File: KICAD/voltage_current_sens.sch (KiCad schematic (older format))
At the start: 22 parts

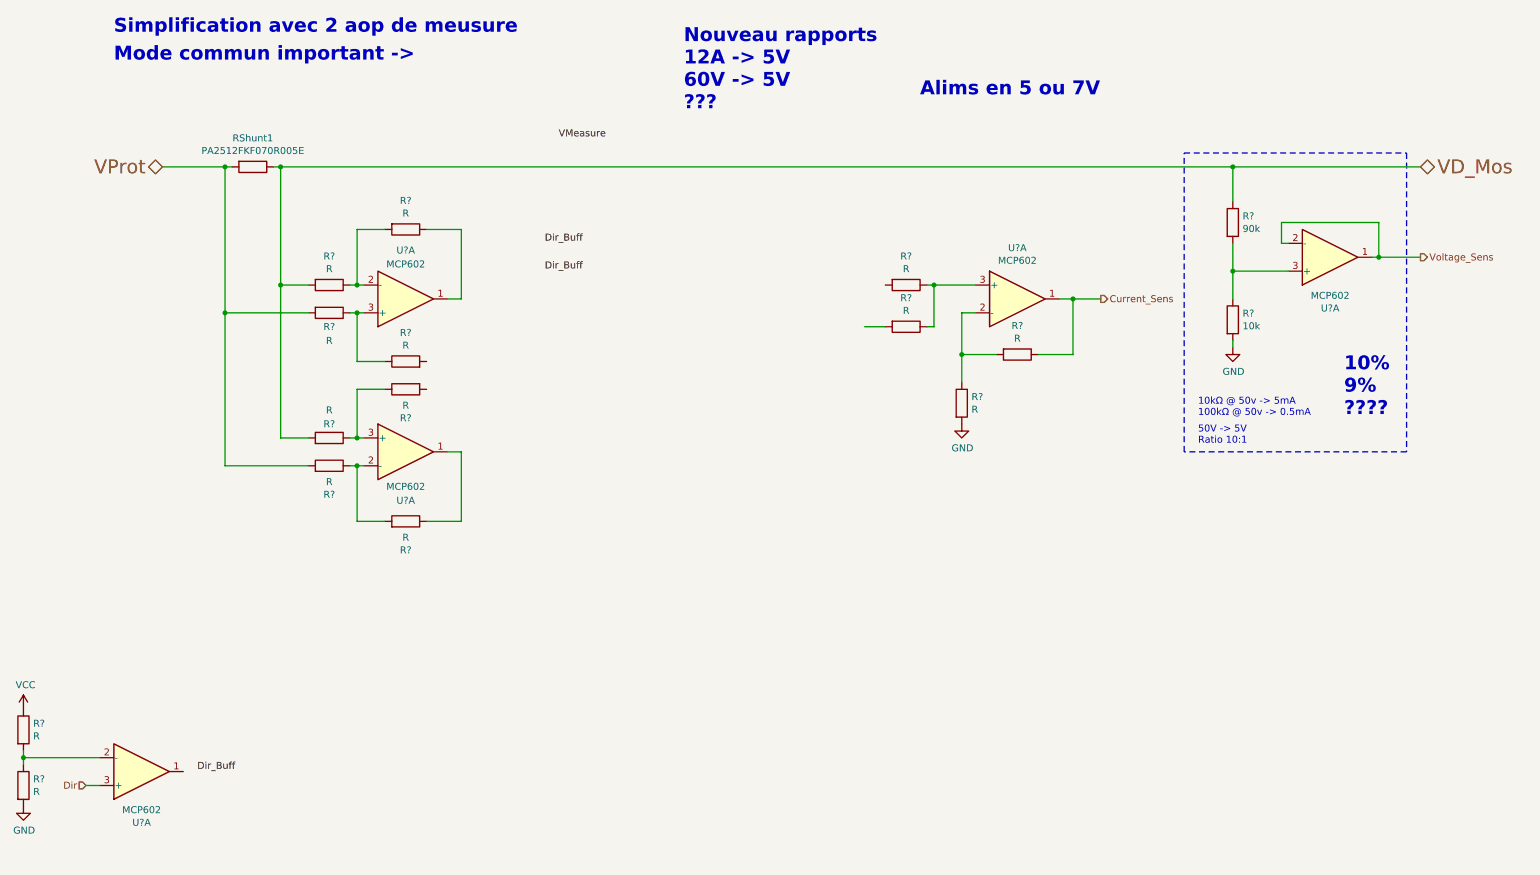
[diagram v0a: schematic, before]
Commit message: worked on power supply + connectors
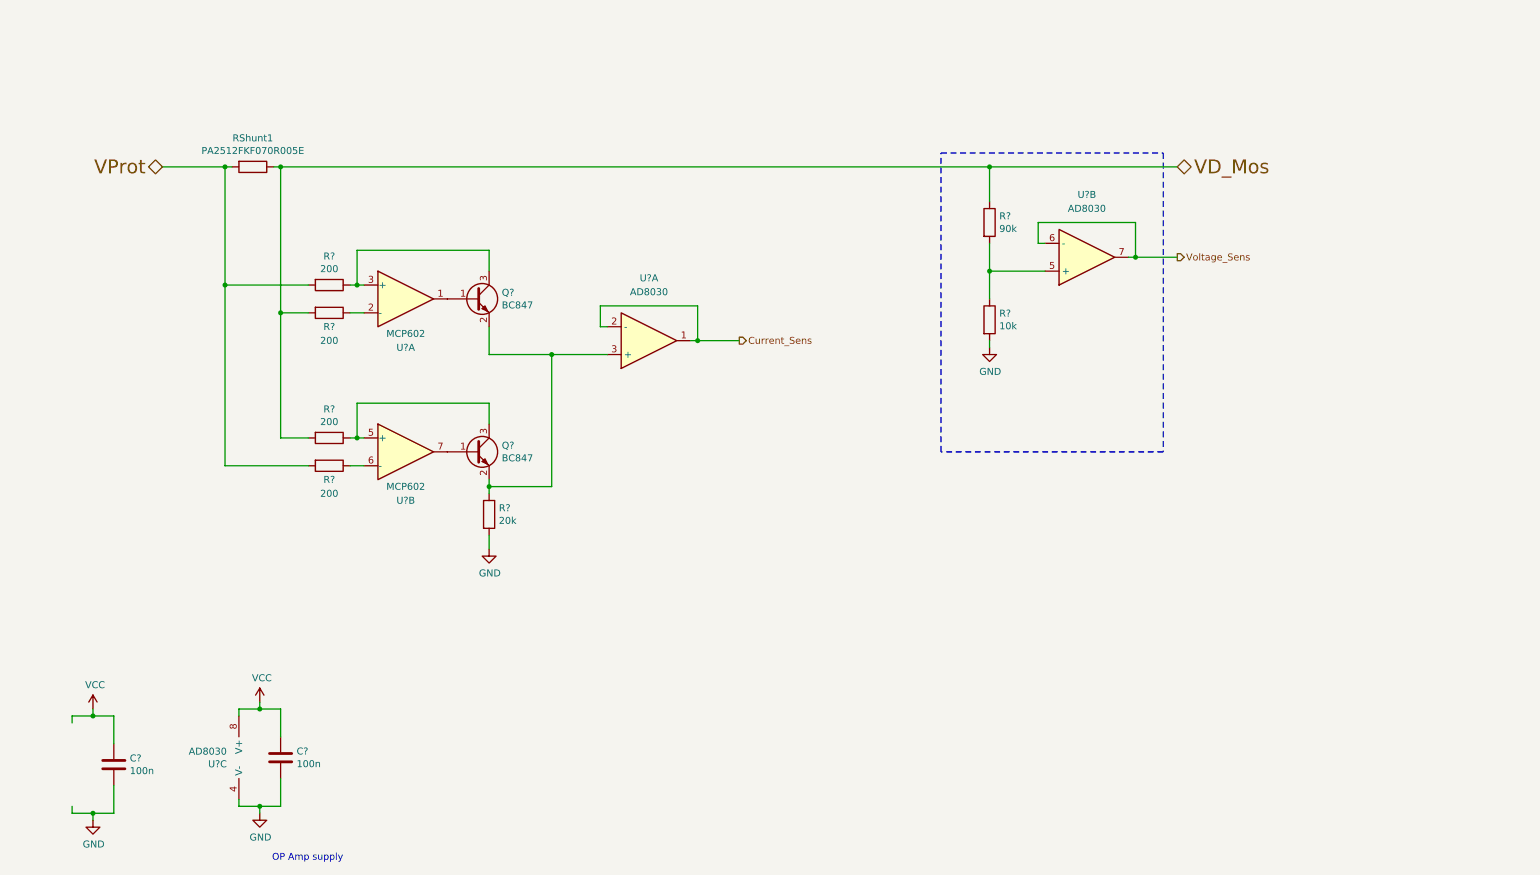
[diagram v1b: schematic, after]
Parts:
- removed R? (x12): R, symbol Device:R
- removed U? (x4): MCP602, symbol Amplifier_Operational:MCP602
- added C? (x2): 100n, symbol Device:C
- added Q? (x2): BC847, Package_TO_SOT_SMD:SOT-23, symbol Transistor_BJT:BC847
- added R?: 20k, symbol Device:R
- added R? (x2): 200, symbol Device:R
- added U?: MCP602, symbol Amplifier_Operational:MCP602
- added U? (x3): AD8030, symbol Sesame:AD8030
- R? (x2): value R -> 200
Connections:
- net labels removed: Dir, Dir_Buff, VMeasure
- wire segments 63 -> 70
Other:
- note added: "OP Amp supply"
- note removed: "10%\n9%\n????"
- note removed: "10kΩ @ 50v -> 5mA\n100kΩ @ 50v -> 0.5mA"
- note removed: "50V -> 5V\nRatio 10:1"
- note removed: "Alims en 5 ou 7V"
- note removed: "Mode commun important ->"
- note removed: "Nouveau rapports\n12A -> 5V\n60V -> 5V\n???"
- note removed: "Simplification avec 2 aop de meusure"
- moved on the sheet: R?
